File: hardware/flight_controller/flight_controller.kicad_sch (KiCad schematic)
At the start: 48 parts, among them J1 Conn_01x02_Pin, U1 BQ25883RGER, U2 TPS63070RNMR, U3 LMR51430XDDCR, U4 BMP581, U5 ICM-45686

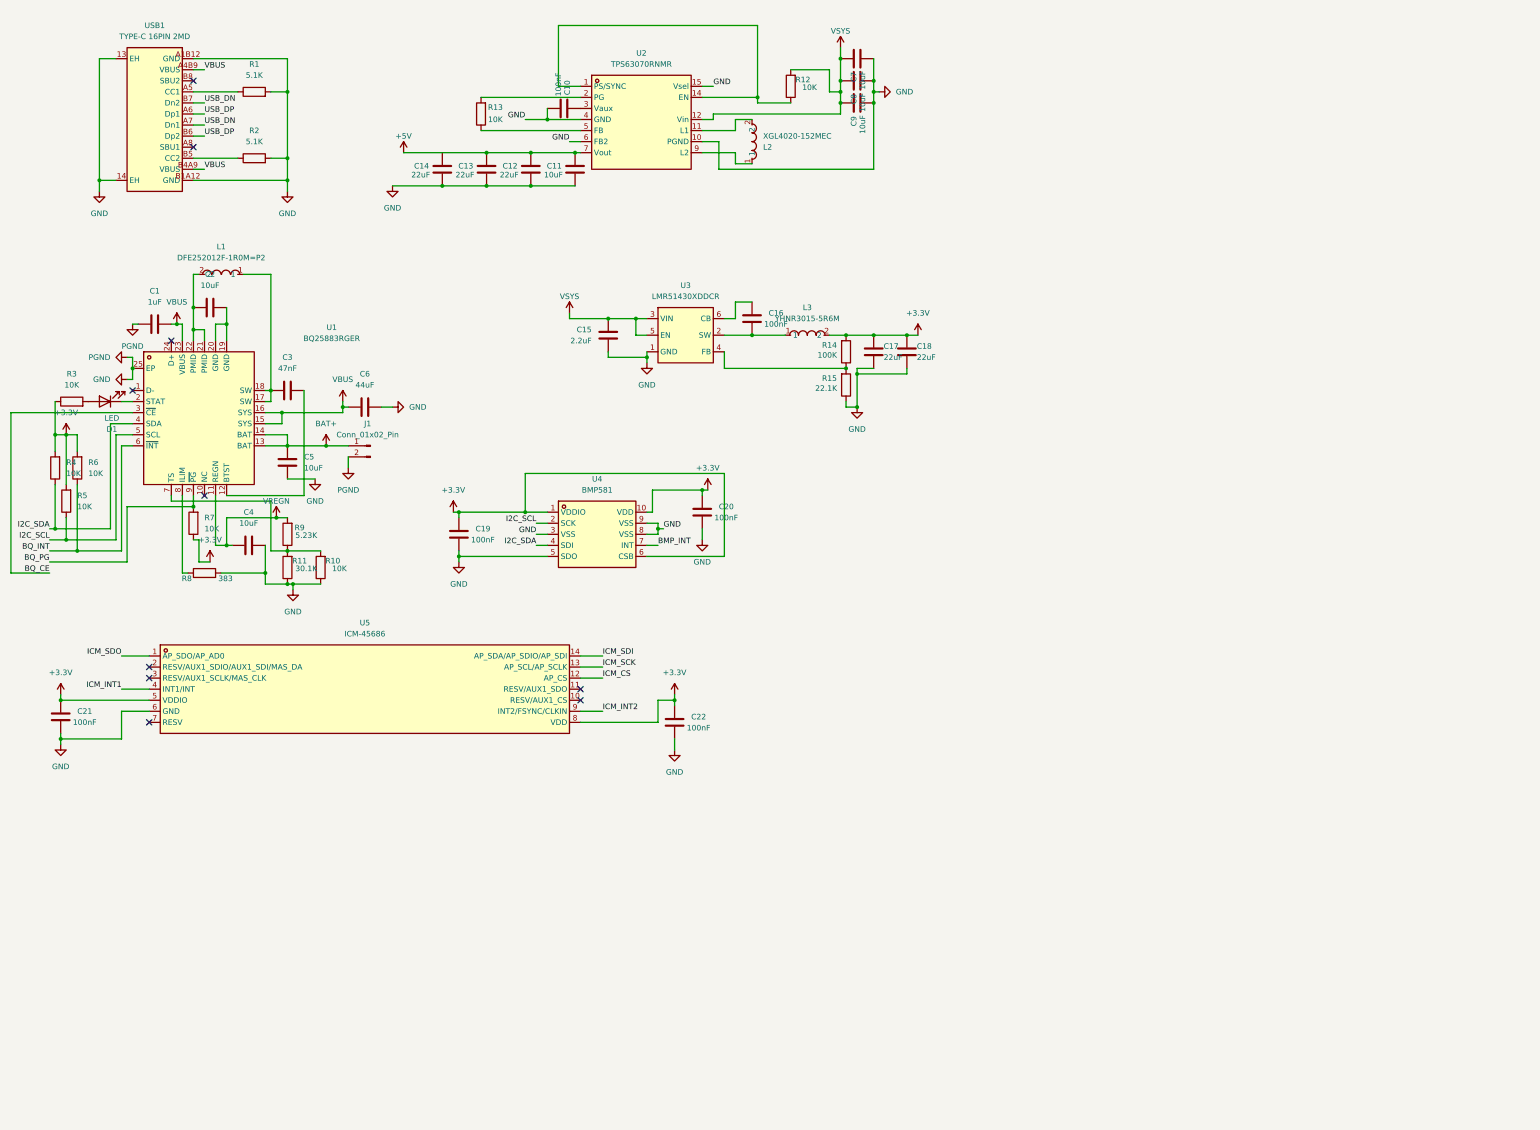
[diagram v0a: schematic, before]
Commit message: GPS, MicroSD, and Magnetometer
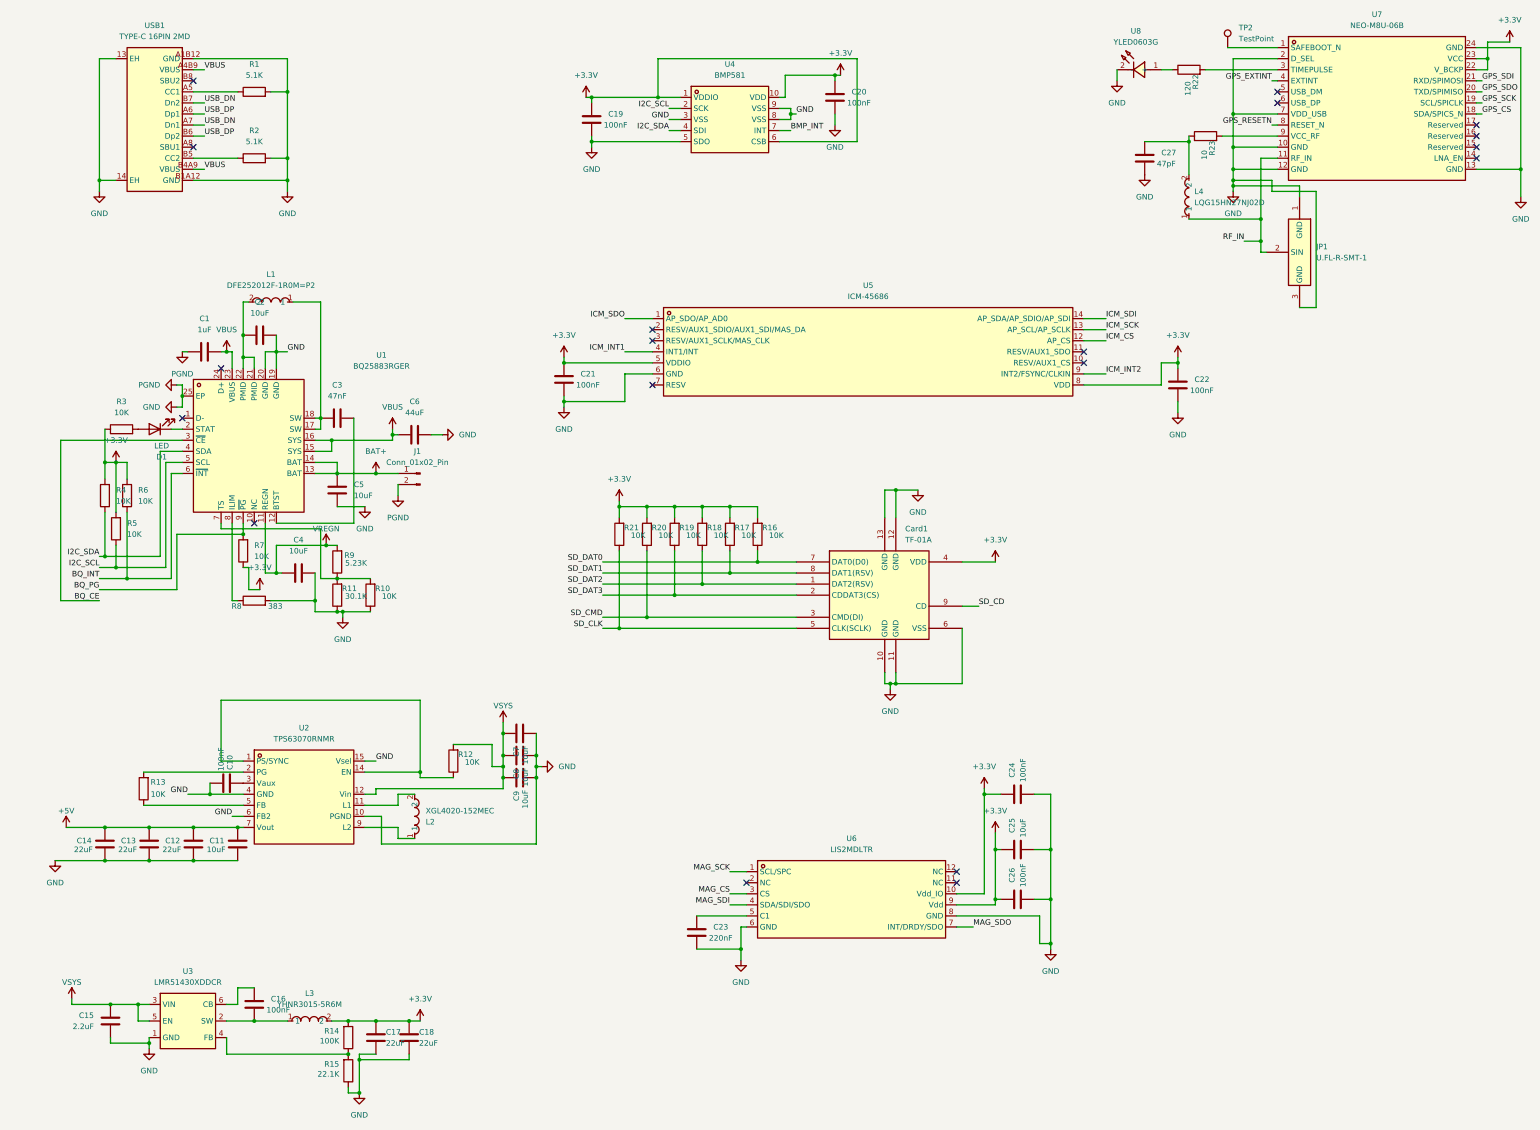
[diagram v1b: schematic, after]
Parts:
- added C23: 220nF, Capacitor_SMD:C_0201_0603Metric, symbol Device:C
- added C24, C26: 100nF, Capacitor_SMD:C_0201_0603Metric, symbol Device:C
- added C25: 10uF, Capacitor_SMD:C_0201_0603Metric, symbol Device:C
- added C27: 47pF, Capacitor_SMD:C_0201_0603Metric, symbol Device:C
- added Card1: TF-01A, easyeda2kicad:TF-SMD_TF-01A, symbol easyeda2kicad:TF-01A
- added JP1: U.FL-R-SMT-1, easyeda2kicad:ANT-SMD_UFL-R-SMT-1-10, symbol easyeda2kicad:U.FL-R-SMT-1
- added L4: LQG15HN27NJ02D, easyeda2kicad:L0402, symbol easyeda2kicad:LQG15HN27NJ02D
- added R16, R17, R18, R19, R20, R21: 10K, Resistor_SMD:R_0201_0603Metric, symbol Device:R
- added R22: 120, Resistor_SMD:R_0201_0603Metric, symbol Device:R
- added R23: 10, Resistor_SMD:R_0201_0603Metric, symbol Device:R
- added TP2: TestPoint, symbol Connector:TestPoint
- added U6: LIS2MDLTR, easyeda2kicad:VLGA-12_L2.0-W2.0-P0.50-BL, symbol easyeda2kicad:LIS2MDLTR
- added U7: NEO-M8U-06B, easyeda2kicad:GPSM-SMD_24P-L16.0-W12.2-P1.10-TL, symbol easyeda2kicad:NEO-M8U-06B
- added U8: YLED0603G, easyeda2kicad:LED0603-FD, symbol easyeda2kicad:YLED0603G
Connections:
- net +3.3V: now also C24.1, C25.1, C26.1, Card1.4 (VDD), R16.2, R17.2, R18.2, R19.2, R20.2, R21.2, U6.10 (Vdd_IO), U6.9 (Vdd), U7.22 (V_BCKP), U7.23 (VCC)
- net +5V: now also C14.1
- net GND: now also C2.2, U1.19 (GND), U1.20 (GND), C23.2, C24.2, C25.2, C26.2, C27.2, Card1.10 (GND), Card1.11 (GND), Card1.12 (GND), Card1.13 (GND), Card1.6 (VSS), JP1.1 (GND), JP1.3 (GND), U6.6 (GND), U6.8 (GND), U7.10 (GND), U7.12 (GND), U7.13 (GND), U7.2 (D_SEL), U7.24 (GND), U7.7 (VDD_USB), U8.2 (-)
- new net: C23.1, U6.5 (C1)
- new net: R22.1, U8.1 (+)
- new net: R22.2, U7.3 (TIMEPULSE)
- new net: C27.1, L4.2, R23.1
- new net: R23.2, U7.9 (VCC_RF)
- new net: TP2.1, U7.1 (SAFEBOOT_N)
- new net GPS_CS: U7.18 (SDA/SPICS_N)
- new net GPS_EXTINT: U7.4 (EXTINT)
- new net GPS_RESETN: U7.8 (RESET_N)
- new net GPS_SCK: U7.19 (SCL/SPICLK)
- new net GPS_SDI: U7.21 (RXD/SPIMOSI)
- new net GPS_SDO: U7.20 (TXD/SPIMISO)
- new net MAG_CS: U6.3 (CS)
- new net MAG_SCK: U6.1 (SCL/SPC)
- new net MAG_SDI: U6.4 (SDA/SDI/SDO)
- new net MAG_SDO: U6.7 (INT/DRDY/SDO)
- new net RF_IN: JP1.2 (SIN), L4.1, U7.11 (RF_IN)
- new net SD_CD: Card1.9 (CD)
- new net SD_CLK: Card1.5 (CLK(SCLK)), R21.1
- new net SD_CMD: Card1.3 (CMD(DI)), R20.1
- new net SD_DAT0: Card1.7 (DAT0(D0)), R16.1
- new net SD_DAT1: Card1.8 (DAT1(RSV)), R17.1
- new net SD_DAT2: Card1.1 (DAT2(RSV)), R18.1
- new net SD_DAT3: Card1.2 (CDDAT3(CS)), R19.1
- no-connect marks 10 -> 19
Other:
- moved on the sheet: C1, C10, C11, C12, C13, C14, C15, C16, C17, C18, C19, C2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
